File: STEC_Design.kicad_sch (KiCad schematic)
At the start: 14 parts, among them Q1 IRLB3034PBF, Q2 IRLB3034PBF, SW1 SW_Push, SW2 SW_Push, U1 L7805CV, U2 MLX90614ESF-BAA-000-TU, U3 ESP32-WROOM-32E, U4 ESP32-DEVKITC-32E

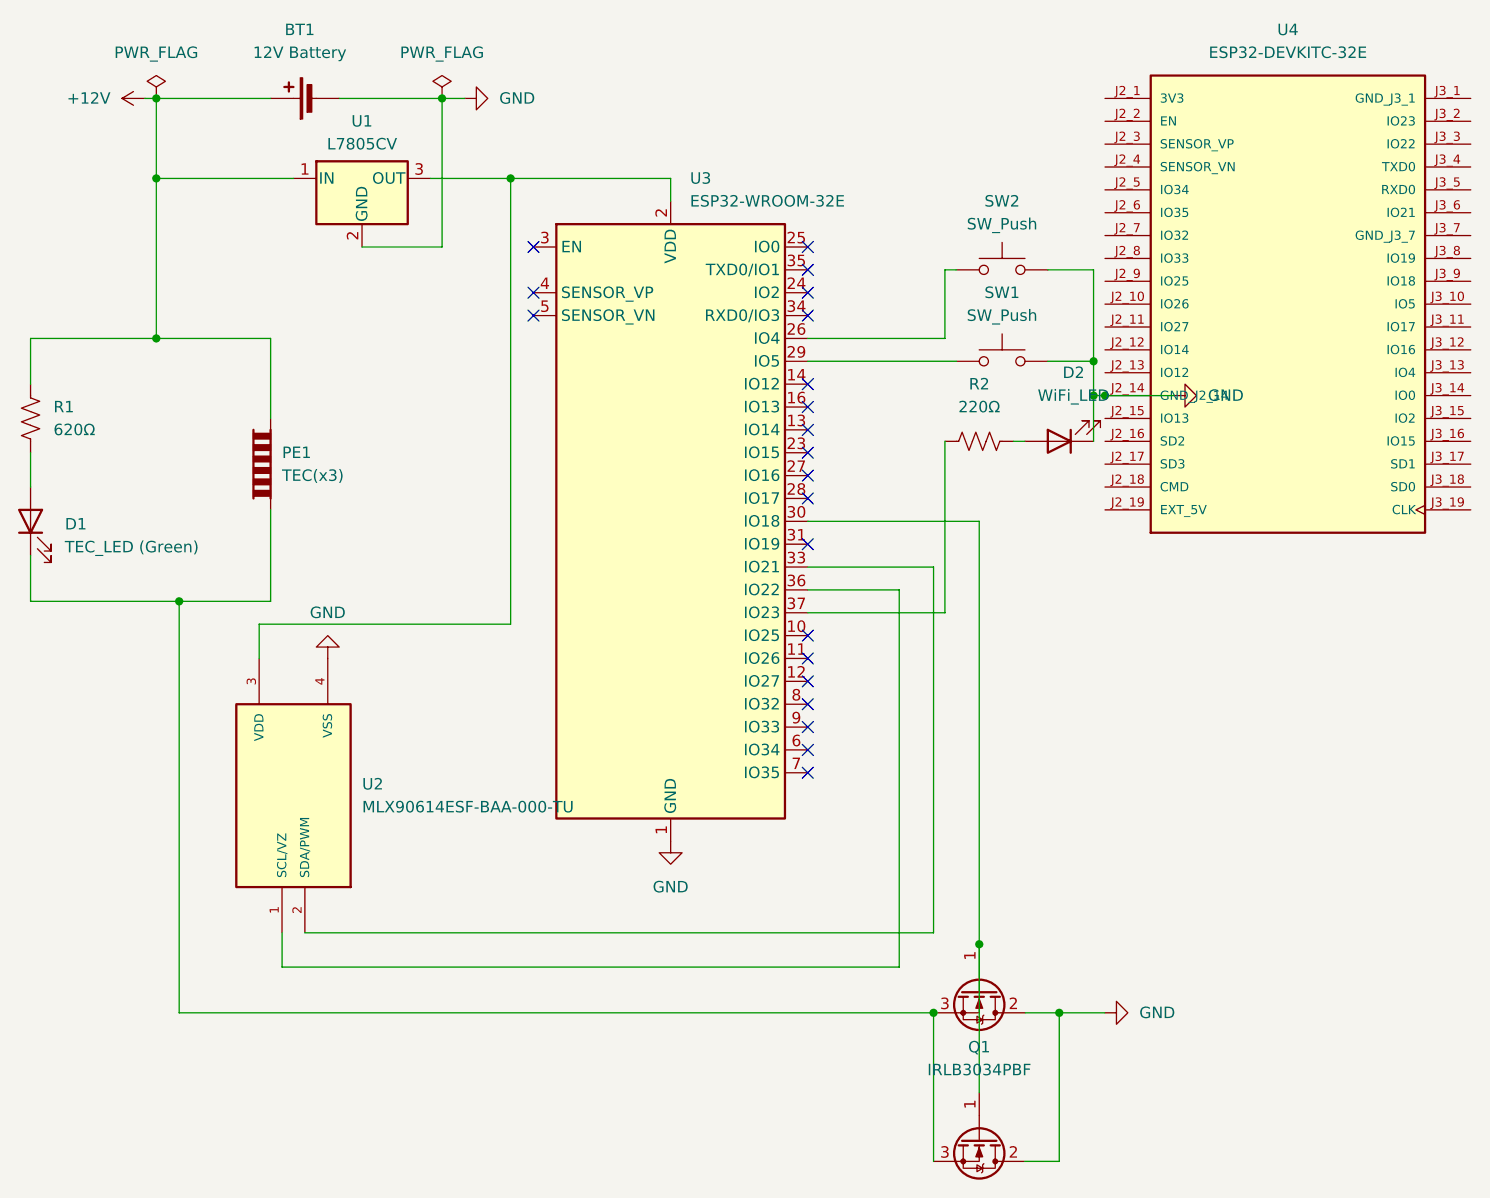
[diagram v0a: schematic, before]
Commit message: finalisedSchematics
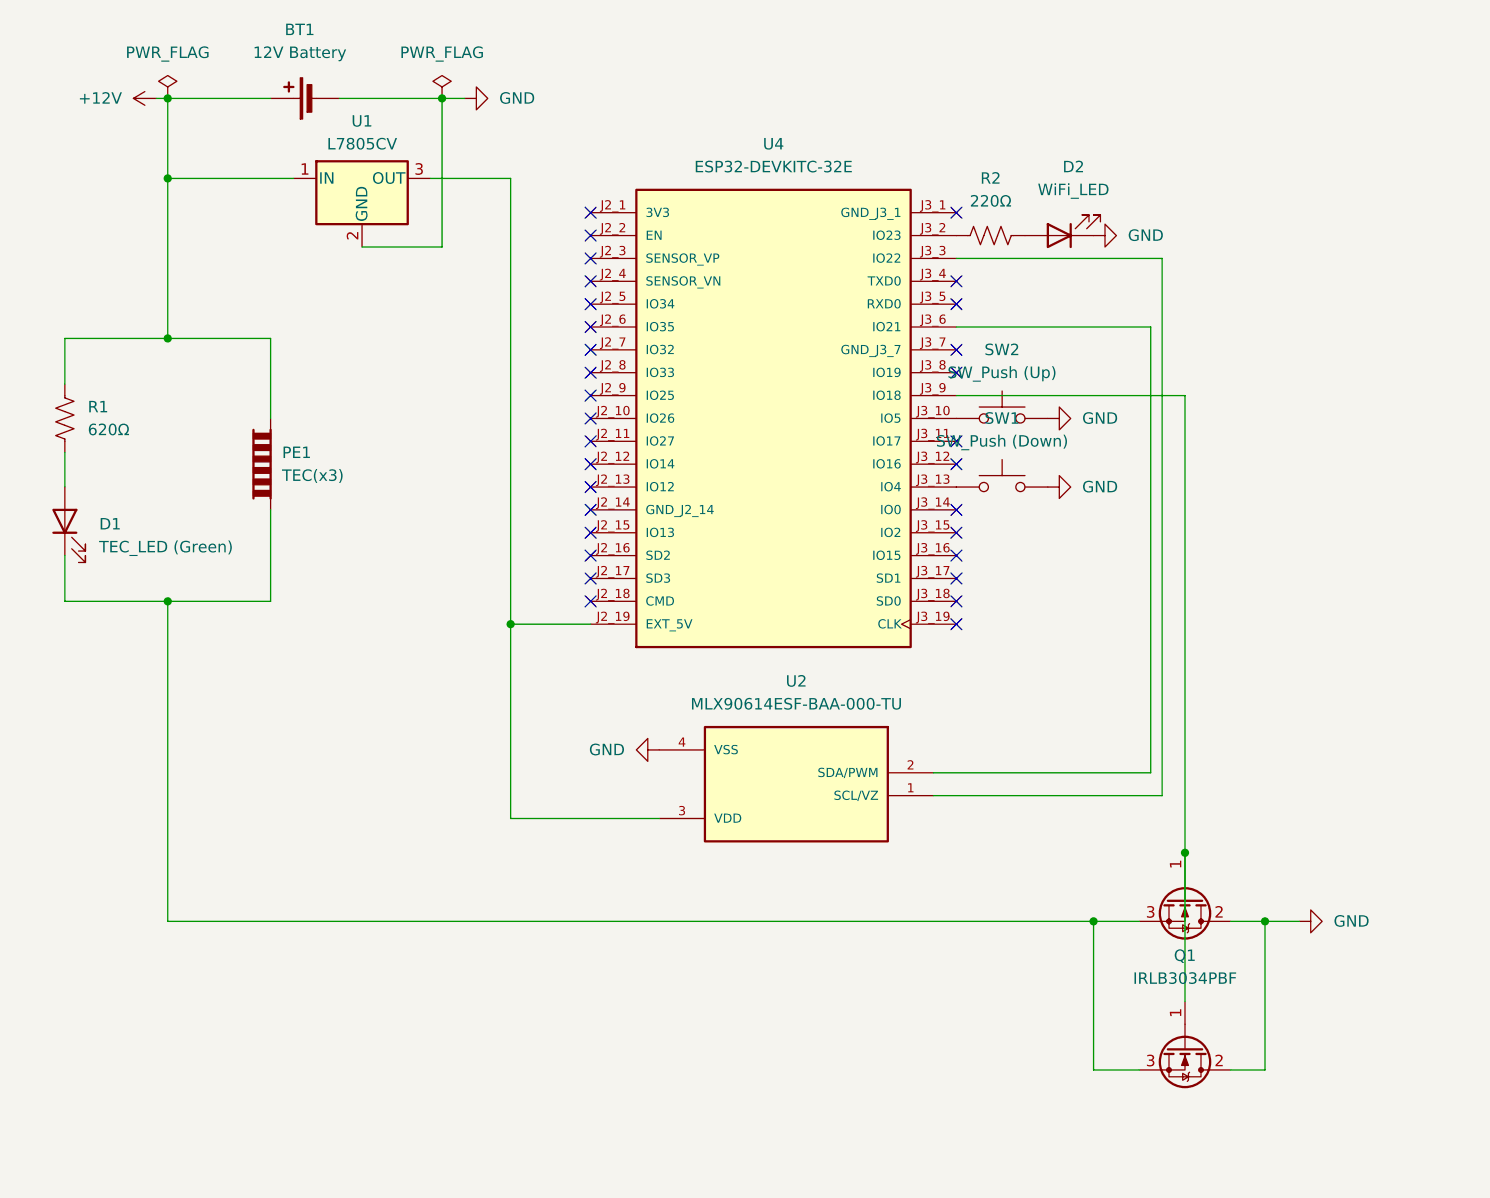
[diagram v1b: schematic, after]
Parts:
- removed U3: ESP32-WROOM-32E, RF_Module:ESP32-WROOM-32D, symbol RF_Module:ESP32-WROOM-32E
- SW1: value SW_Push -> SW_Push (Down)
- SW2: value SW_Push -> SW_Push (Up)
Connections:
- net GND: no longer U4.J2_14 (GND_J2_14)
- net at U1.3 (OUT), U2.3 (VDD): now also U4.J2_19 (EXT_5V)
- net at SW1.1: now also U4.J3_13 (IO4)
- net at SW2.1: now also U4.J3_10 (IO5)
- net at Q1.1 (G), Q2.1 (G): now also U4.J3_9 (IO18)
- net at U2.2 (SDA/PWM): now also U4.J3_6 (IO21)
- net at U2.1 (SCL/VZ): now also U4.J3_3 (IO22)
- net at R2.2: now also U4.J3_2 (IO23)
- no-connect marks 21 -> 31
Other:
- moved on the sheet: D1, D2, Q1, R1, R2, SW1, SW2, U2, U4
